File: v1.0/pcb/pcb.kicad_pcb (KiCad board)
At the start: 2 copper layers, 375 x 125 mm, 323 parts, among them J1 USB_C_Receptacle_USB2.0, J2 ISP, SW1 SW_Push, SW10 SW_Push, SW11 SW_Push, SW12 SW_Push, SW13 SW_Push, SW14 SW_Push, SW15 SW_Push, SW16 SW_Push, SW17 SW_Push, SW18 SW_Push, SW19 SW_Push, SW2 SW_Push, SW20 SW_Push, SW21 SW_Push, SW22 SW_Push, SW23 SW_Push, SW24 SW_Push, SW25 SW_Push, SW26 SW_Push, SW27 SW_Push, SW28 SW_Push, SW29 SW_Push, SW3 SW_Push, SW30 SW_Push, SW31 SW_Push, SW32 SW_Push, SW33 SW_Push, SW34 SW_Push, SW35 SW_Push, SW36 SW_Push, SW37 SW_Push, SW38 SW_Push, SW39 SW_Push, SW4 SW_Push, SW40 SW_Push, SW41 SW_Push, SW42 SW_Push, SW43 SW_Push, SW44 SW_Push, SW45 SW_Push, SW46 SW_Push, SW47 SW_Push, SW48 SW_Push, SW49 SW_Push, SW5 SW_Push, SW50 SW_Push, SW51 SW_Push, SW52 SW_Push, SW53 SW_Push, SW54 SW_Push, SW55 SW_Push, SW56 SW_Push, SW57 SW_Push, SW58 SW_Push, SW59 SW_Push, SW6 SW_Push, SW60 SW_Push, SW61 SW_Push, SW62 SW_Push, SW63 SW_Push, SW64 SW_Push, SW65 SW_Push, SW66 SW_Push, SW67 SW_Push, SW68 SW_Push, SW69 SW_Push, SW7 SW_Push, SW70 SW_Push, SW71 SW_Push, SW72 SW_Push, SW73 SW_Push, SW74 SW_Push, SW75 SW_Push, SW76 SW_Push, SW77 SW_Push, SW78 SW_Push, SW79 SW_Push, SW8 SW_Push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

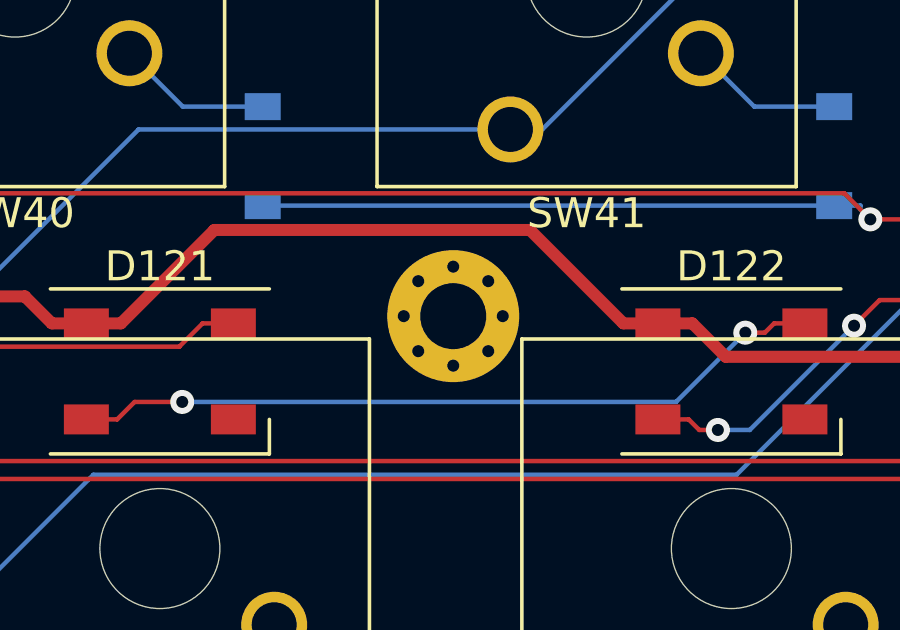
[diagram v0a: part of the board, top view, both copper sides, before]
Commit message: software changes
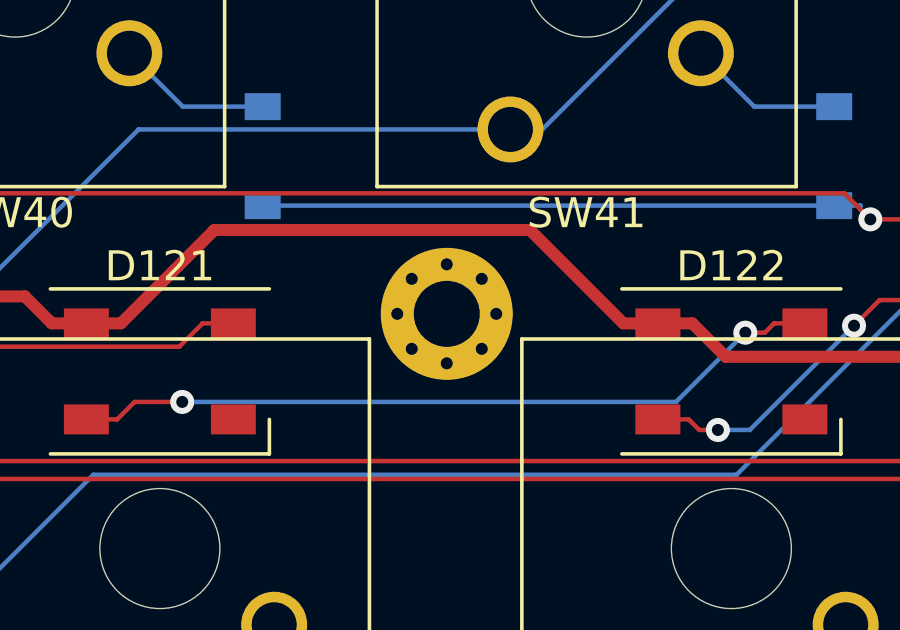
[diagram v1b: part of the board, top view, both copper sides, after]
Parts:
- moved H10 0.23 mm to (174.5, 183.8)
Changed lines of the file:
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@@
   )
   (module MountingHole:MountingHole_2.2mm_M2_Pad_Via (layer F.Cu)
-    (at 174.6885 183.896)
+    (at 174.4726 183.8198)
     (descr "Mounting Hole 2.2mm, M2")
     (tags "mounting hole 2.2mm m2")
